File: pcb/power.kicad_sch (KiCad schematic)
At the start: 13 parts, among them J6 USB_C_Receptacle_USB2.0_16P, J7 Raspberry_Pi_4, U4 AMS1117-3.3, U9 TPS5430DDA

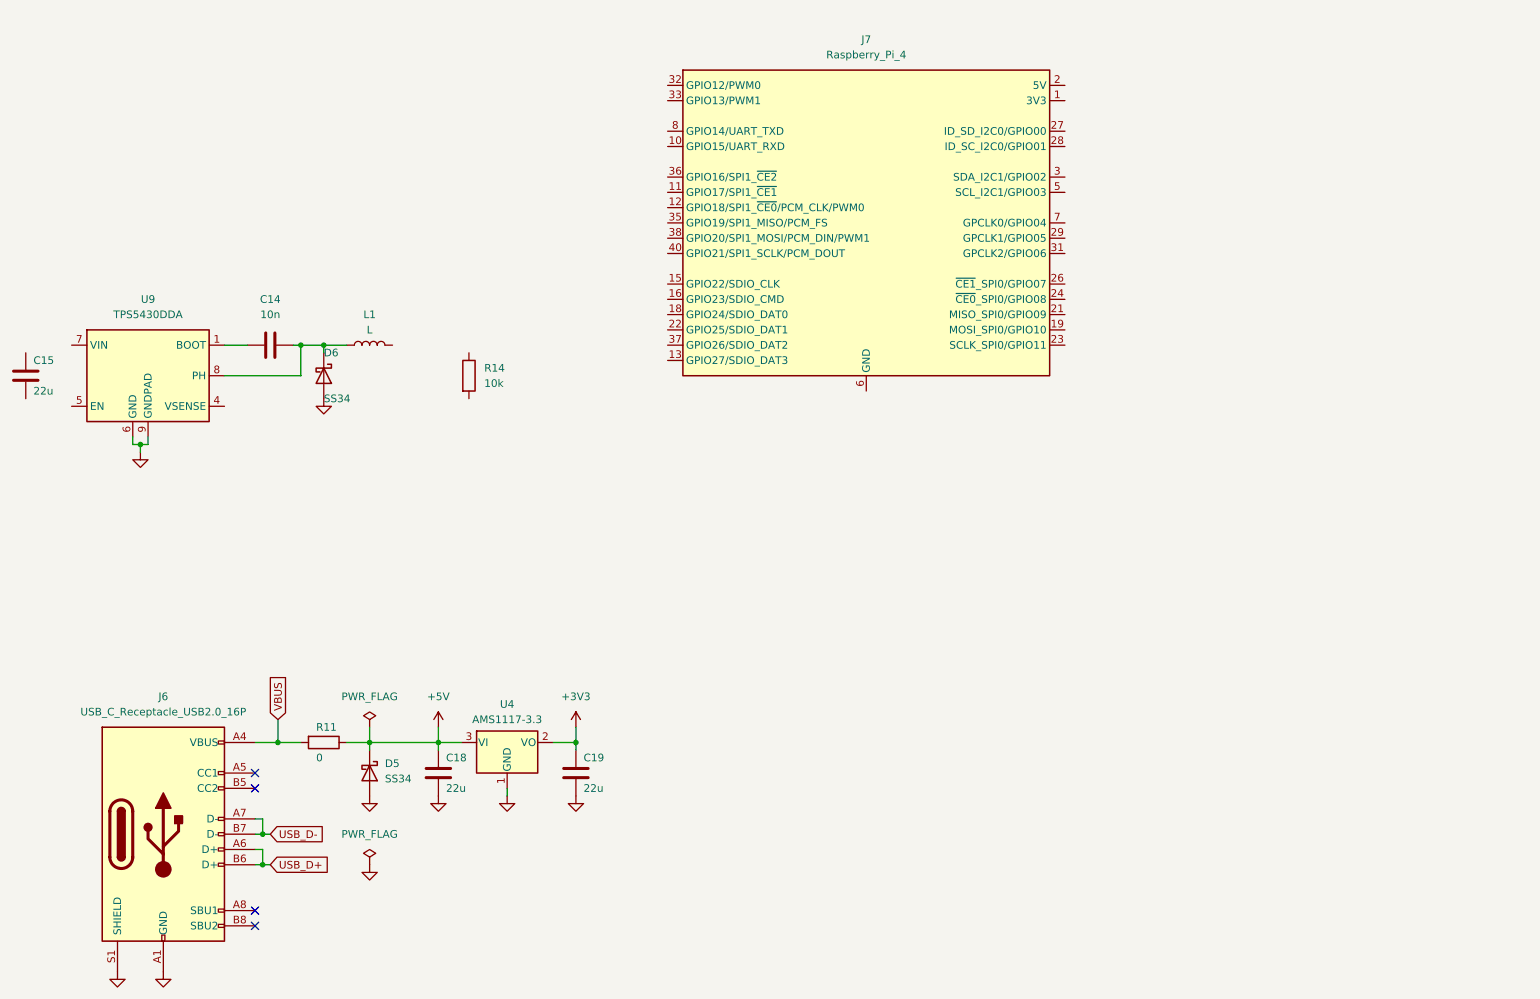
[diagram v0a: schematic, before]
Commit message: WIP on the motor driver board
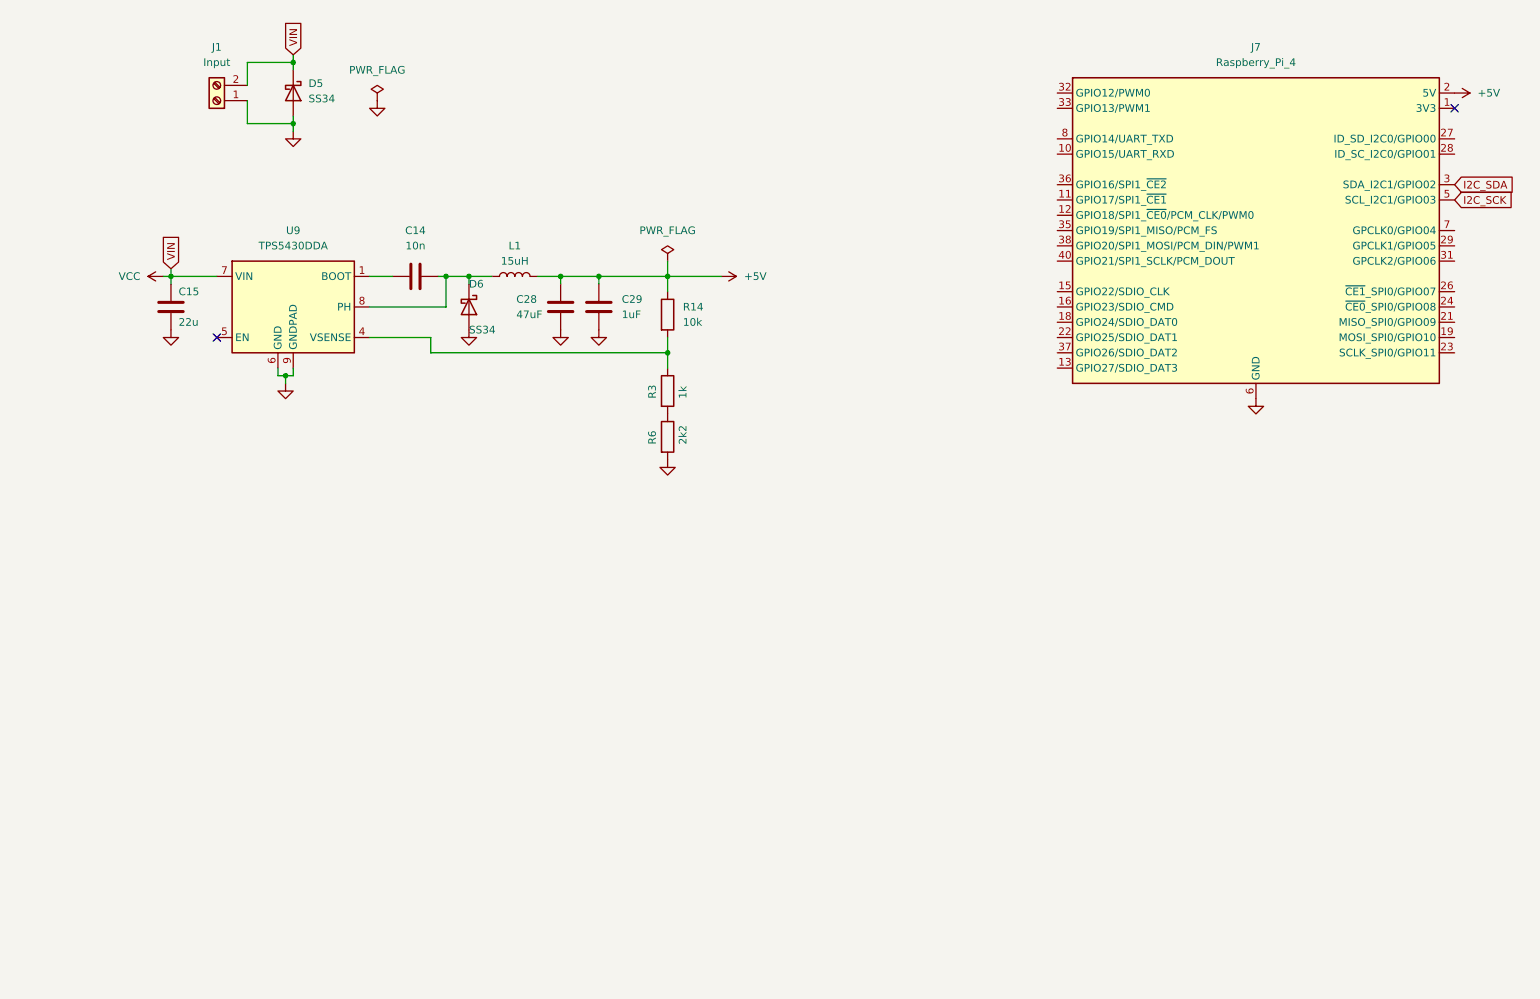
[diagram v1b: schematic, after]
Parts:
- removed C18, C19: 22u, Capacitor_SMD:C_0805_2012Metric, symbol Device:C
- removed J6: USB_C_Receptacle_USB2.0_16P, Connector_USB:USB_C_Receptacle_G-Switch_GT-USB-7010ASV, symbol Connector:USB_C_Receptacle_USB2.0_16P
- removed R11: 0, Resistor_SMD:R_0603_1608Metric, symbol Device:R
- removed U4: AMS1117-3.3, Package_TO_SOT_SMD:SOT-223, symbol Regulator_Linear:XC6206PxxxMR
- added C28: 47uF, Capacitor_SMD:C_1206_3216Metric, symbol Device:C
- added C29: 1uF, Capacitor_SMD:C_0805_2012Metric, symbol Device:C
- added J1: Input, TerminalBlock_Phoenix:TerminalBlock_Phoenix_MKDS-1,5-2-5.08_1x02_P5.08mm_Horizontal, symbol Connector:Screw_Terminal_01x02
- added R3: 1k, Resistor_SMD:R_0402_1005Metric, symbol Device:R
- added R6: 2k2, Resistor_SMD:R_0402_1005Metric, symbol Device:R
- J7: footprint (none) -> Connector_PinSocket_2.54mm:PinSocket_2x20_P2.54mm_Vertical
- L1: value L -> 15uH; footprint (none) -> Inductor_SMD:L_Changjiang_FXL0630; LCSC Part (none) -> C177243
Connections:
- net +5V: now also J7.2 (5V), J7.4 (5V), L1.2, R14.1, C28.1, C29.1; no longer D5.1 (K)
- net GND: now also C15.2, J7.14 (GND), J7.20 (GND), J7.25 (GND), J7.30 (GND), J7.34 (GND), J7.39 (GND), J7.6 (GND), J7.9 (GND), C28.2, C29.2, J1.1 (Pin_1), R6.2
- net VCC: now reaches C15.1
- net VCC: now also D5.1 (K), U9.7 (VIN), J1.2 (Pin_2)
- net at U9.4 (VSENSE): now also R14.2, R3.1
- net I2C_SDA: now reaches J7.3 (SDA_I2C1/GPIO02)
- net I2C_SCK: now reaches J7.5 (SCL_I2C1/GPIO03)
- new net: R3.2, R6.1
- no-connect marks 4 -> 2
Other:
- moved on the sheet: C14, C15, D5, D6, J7, L1, R14, U9
